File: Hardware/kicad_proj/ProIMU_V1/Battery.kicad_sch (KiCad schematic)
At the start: 30 parts, among them IC1 MP2731GQC-0000-Z, Q1 2SC4213, SW1 SW_SPDT, U7 TPS54308, U8 TPS54308

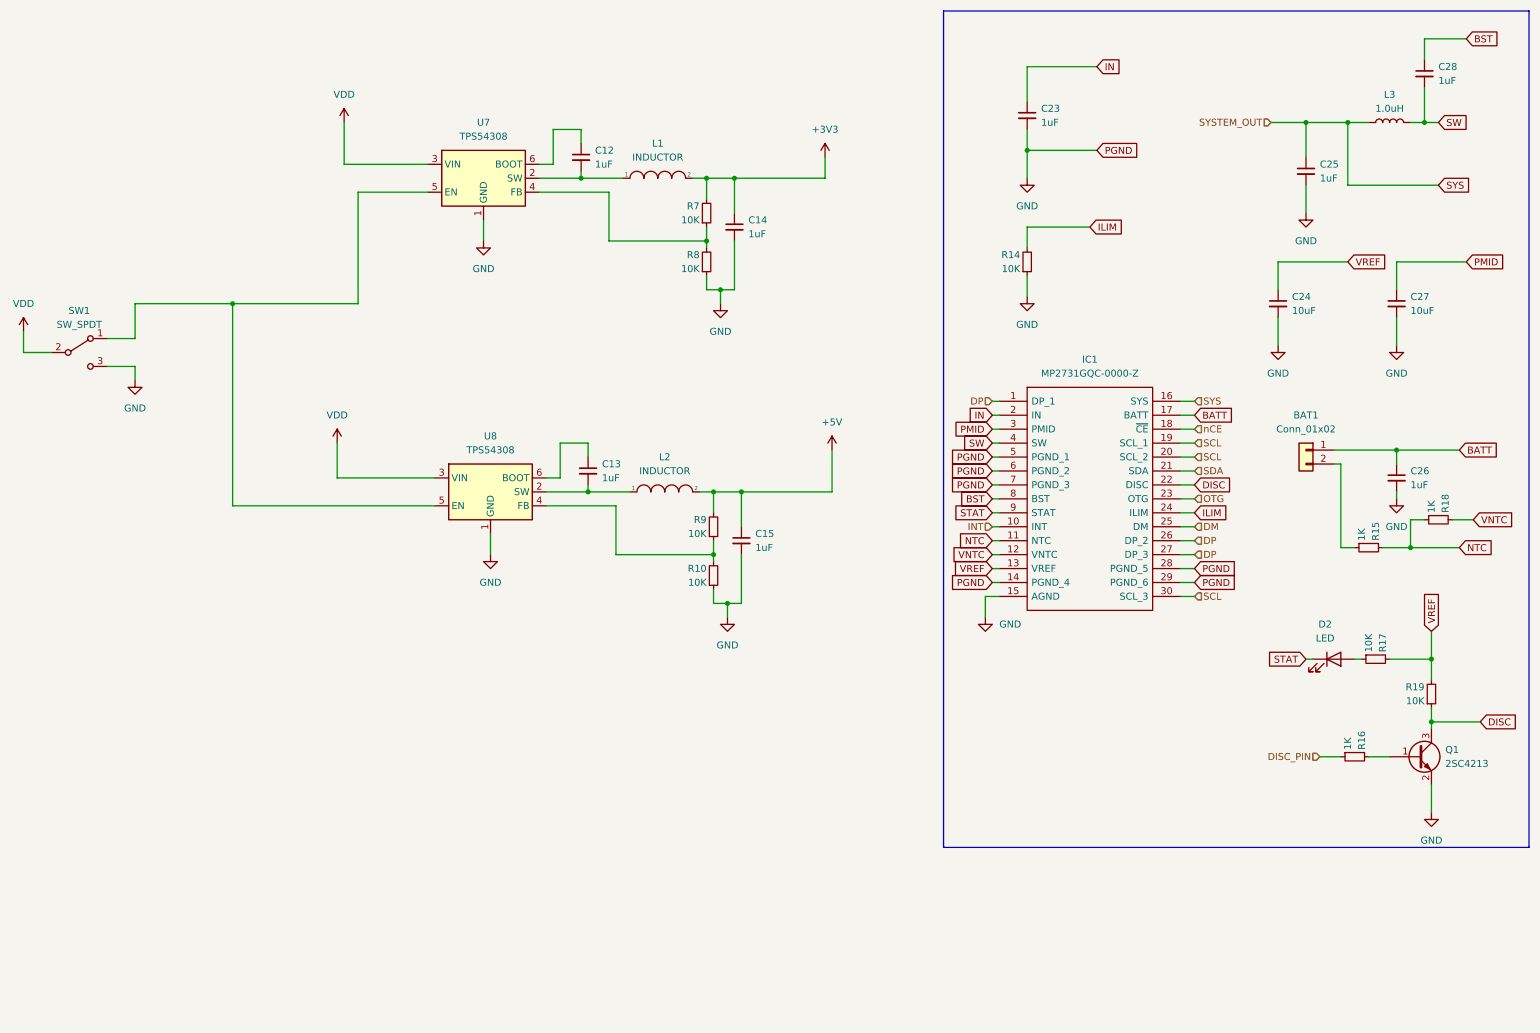
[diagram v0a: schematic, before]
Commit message: Updated Schematic
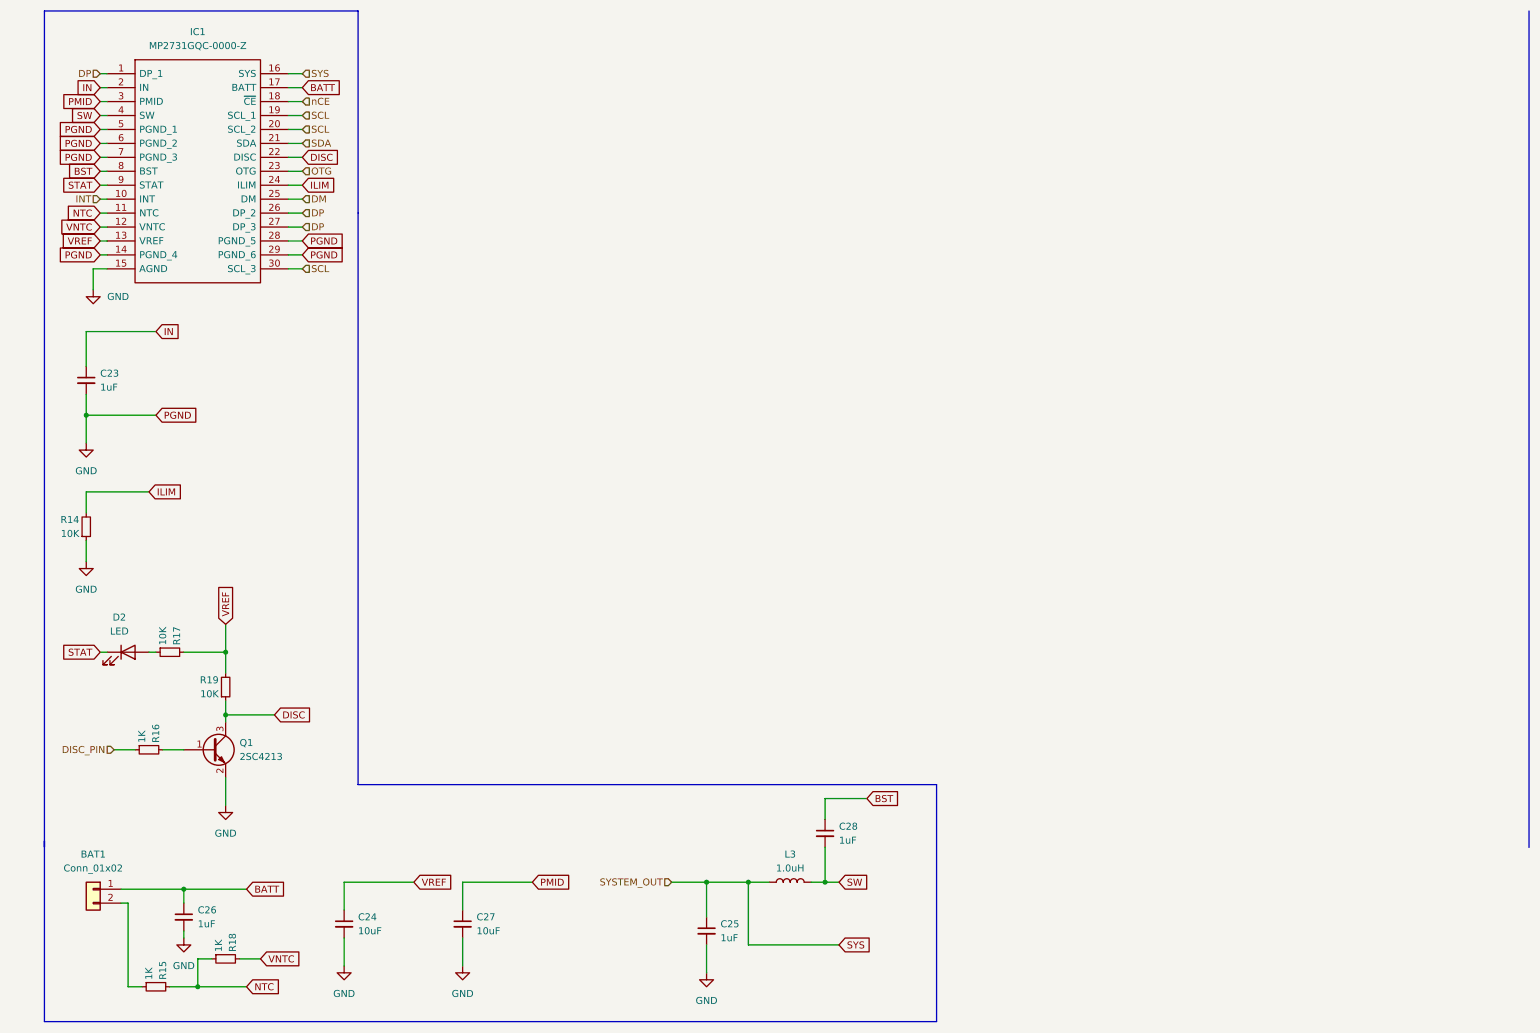
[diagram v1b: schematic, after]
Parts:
- removed C12, C13, C14, C15: 1uF, Capacitor_SMD:C_0402_1005Metric_Pad0.74x0.62mm_HandSolder, symbol Device:C_Small
- removed L1, L2: INDUCTOR, symbol pspice:INDUCTOR
- removed R10, R7, R8, R9: 10K, Resistor_SMD:R_0402_1005Metric_Pad0.72x0.64mm_HandSolder, symbol Device:R_Small
- removed SW1: SW_SPDT, symbol Switch:SW_SPDT
- removed U7, U8: TPS54308, Package_TO_SOT_SMD:SOT-23-6, symbol Regulator_Switching:TPS54308
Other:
- moved on the sheet: BAT1, C23, C24, C25, C26, C27, C28, D2, IC1, L3, Q1, R14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
